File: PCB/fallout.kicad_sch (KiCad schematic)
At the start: 3 parts, among them M1 Motor_DC, U1 VL53L0CXV0DH1, U2 DRV8833PWP

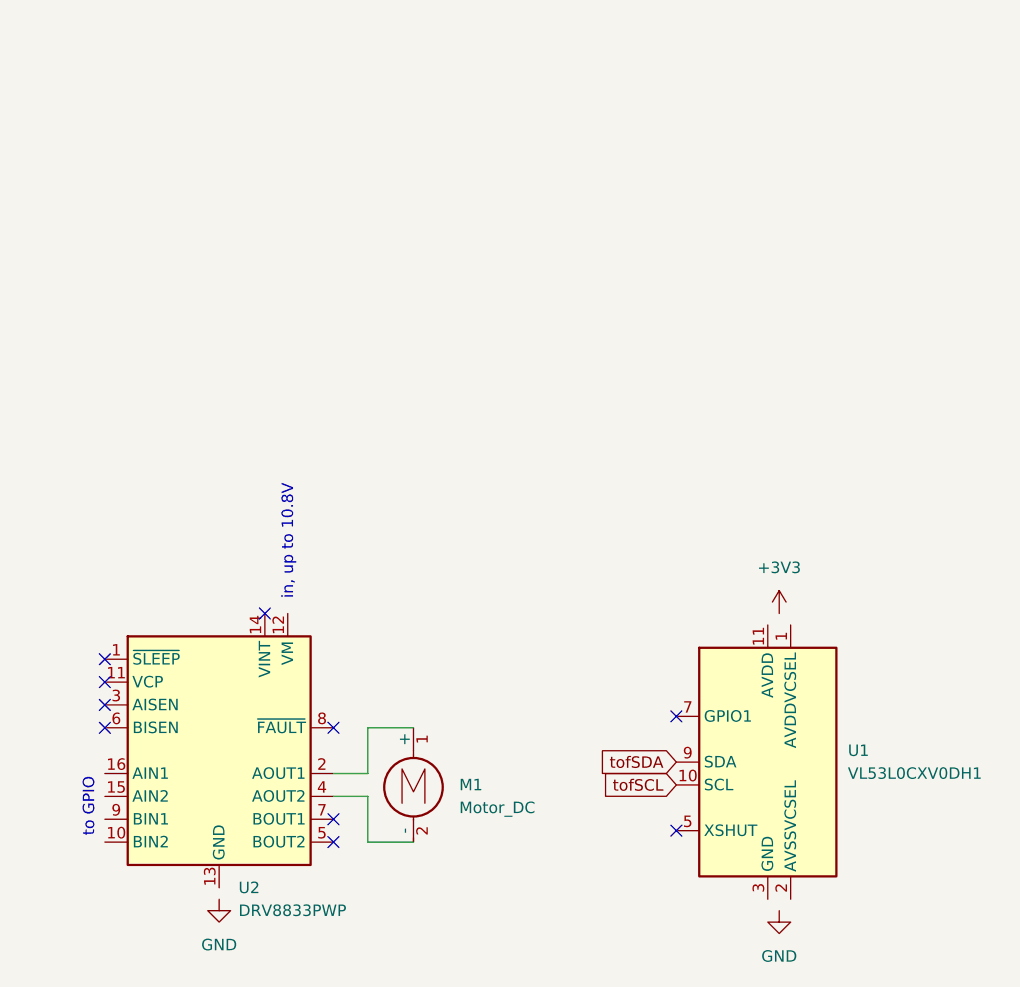
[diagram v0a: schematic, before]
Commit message: update schematics
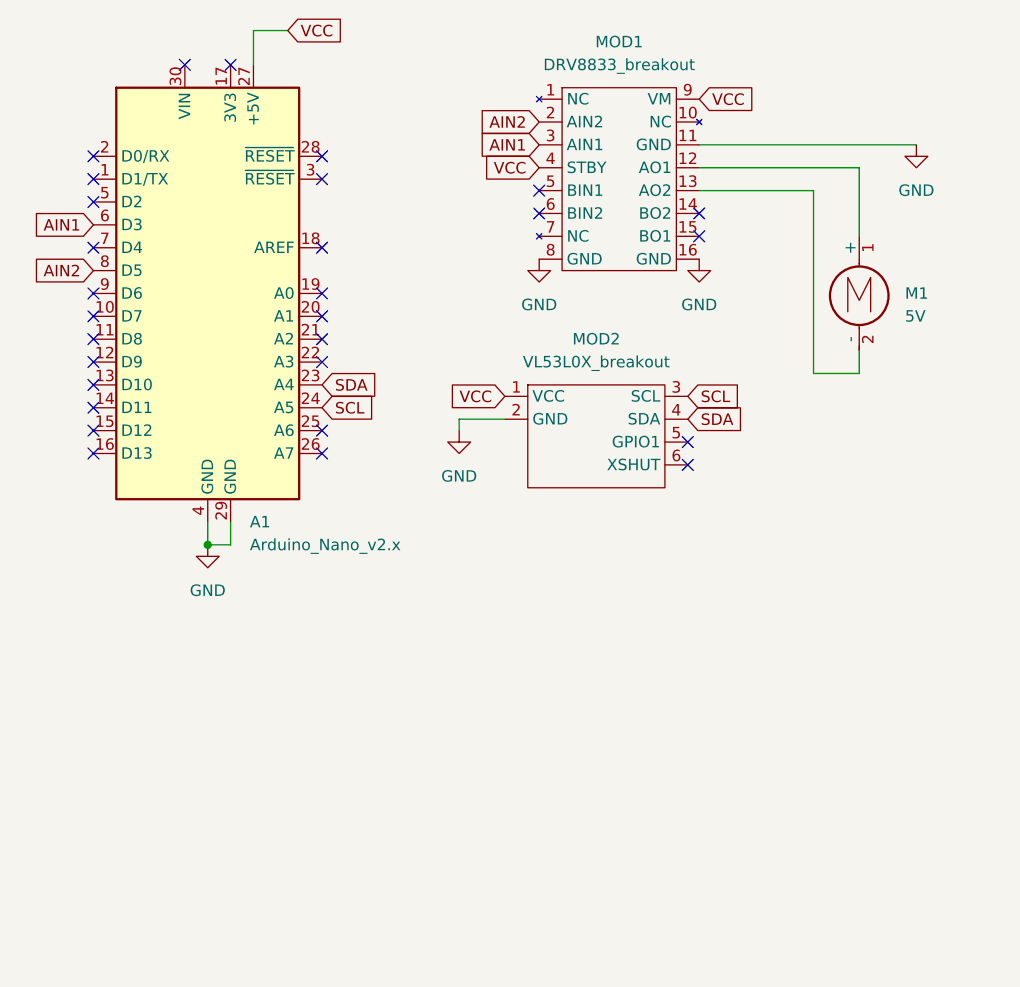
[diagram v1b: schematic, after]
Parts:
- removed U1: VL53L0CXV0DH1, Sensor_Distance:ST_VL53L1x, symbol Sensor_Distance:VL53L0CXV0DH1
- removed U2: DRV8833PWP, Package_SO:HTSSOP-16-1EP_4.4x5mm_P0.65mm_EP3.4x5mm_Mask2.46x2.31mm_ThermalVias, symbol Driver_Motor:DRV8833PWP
- added A1: Arduino_Nano_v2.x, Module:Arduino_Nano, symbol MCU_Module:Arduino_Nano_v2.x
- added MOD1: DRV8833_breakout, symbol Misc_Components:DRV3388_Breakout
- added MOD2: VL53L0X_breakout, symbol Misc_Components:vl53l0x_breakout
- M1: value Motor_DC -> 5V
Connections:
- net GND: now also A1.29 (GND), A1.4 (GND), MOD1.11 (GND), MOD1.16 (GND), MOD1.8 (GND), MOD2.2 (GND)
- net at M1.1 (+): now also MOD1.12 (AO1)
- net at M1.2 (-): now also MOD1.13 (AO2)
- new net AIN1: A1.6 (D3), MOD1.3 (AIN1)
- new net AIN2: A1.8 (D5), MOD1.2 (AIN2)
- new net SCL: A1.24 (A5), MOD2.3 (SCL)
- new net SDA: A1.23 (A4), MOD2.4 (SDA)
- new net VCC: A1.27 (+5V), MOD1.4 (STBY), MOD1.9 (VM), MOD2.1 (VCC)
- no-connect marks 10 -> 29
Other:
- note removed: "in, up to 10.8V"
- note removed: "to GPIO"
